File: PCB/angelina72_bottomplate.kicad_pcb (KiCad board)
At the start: 2 copper layers, 176.4 x 111.6 mm, 45 parts

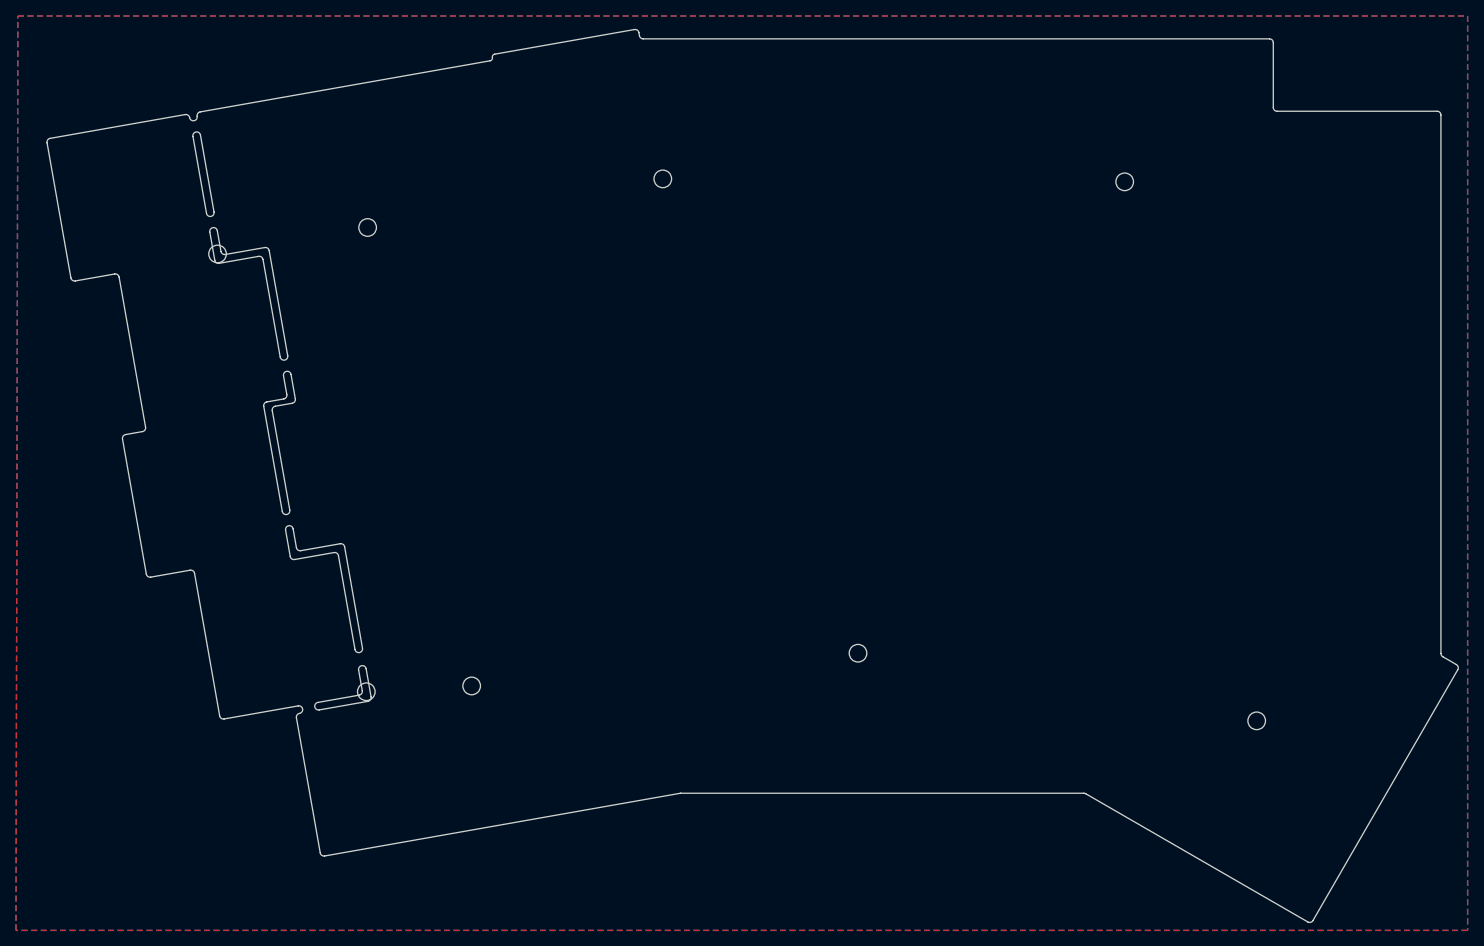
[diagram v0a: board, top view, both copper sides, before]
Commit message: Update PCBs
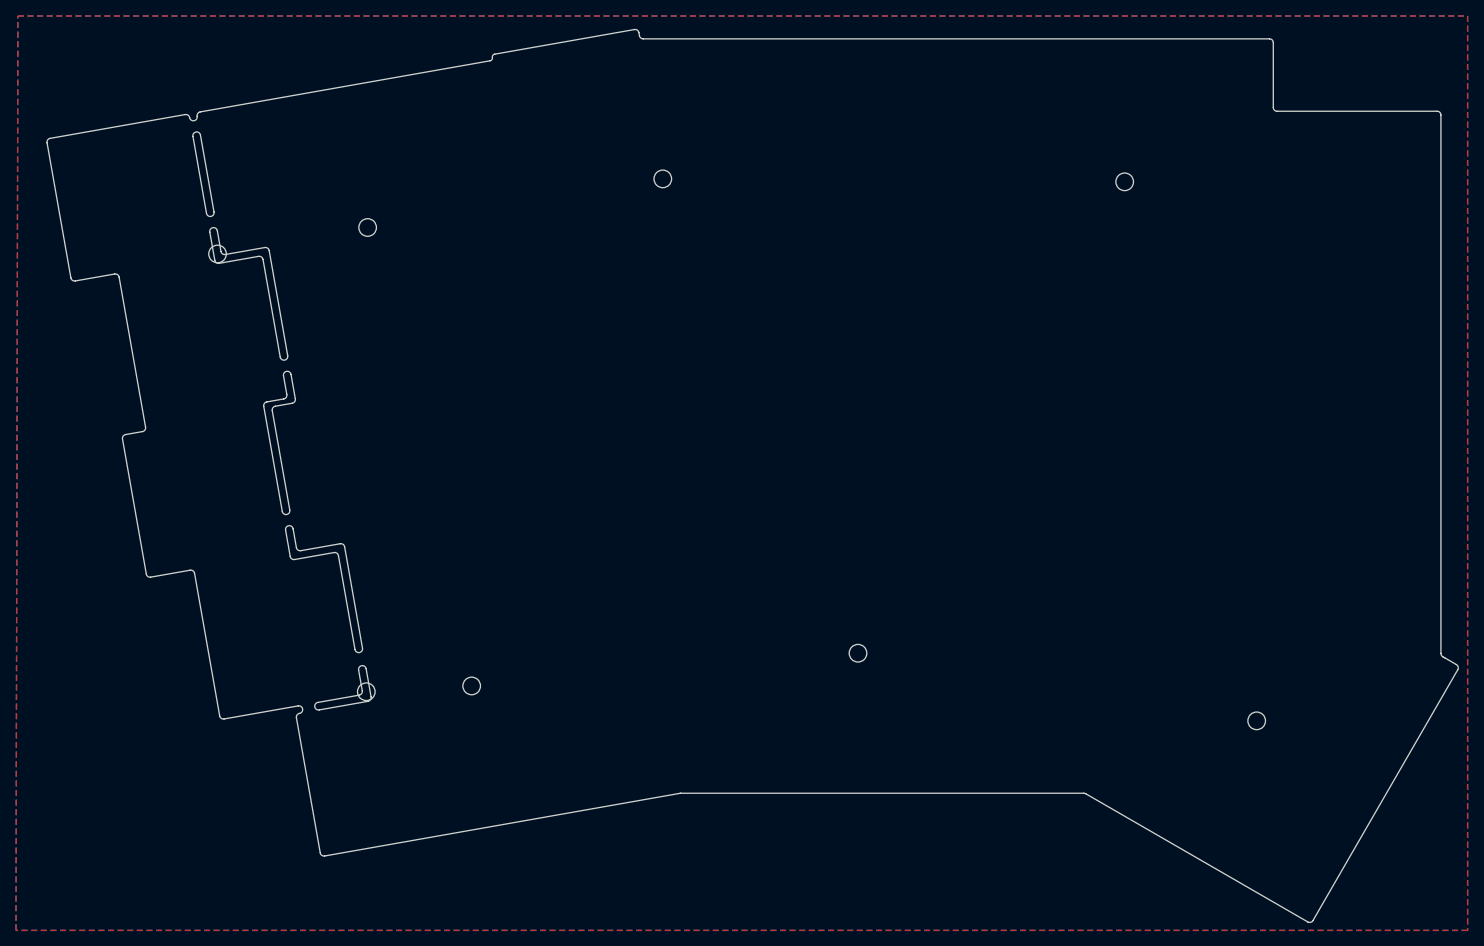
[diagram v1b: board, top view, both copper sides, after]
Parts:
- added REF**: Layout_Outline_PromicroBase, angelina72:Layout_Outline_PromicroBase, F.Cu at (113.2, 113.0)
- added REF**: Layout_Outline, angelina72:Layout_Outline, F.Cu at (113.2, 113.0)
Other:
- outline, holes or cut-outs redrawn
